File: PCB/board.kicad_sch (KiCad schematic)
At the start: 171 parts, among them J1 Micro_SD_Card, J10 Conn_01x10, J11 Conn_01x02, J12 Conn_02x04_Odd_Even, J13 Conn_01x02, J14 Conn_01x02, J15 Conn_01x03, J16 Conn_01x02, J17 Conn_01x05, J18 Conn_01x04, J19 Conn_01x04, J2 Conn_ARM_JTAG_SWD_10, J20 Conn_01x02, J21 Conn_01x03, J22 Conn_02x04_Odd_Even, J23 Conn_01x04, J24 Conn_01x04, J25 Conn_01x02, J26 Conn_01x03, J27 Conn_02x04_Odd_Even, J28 Conn_01x04, J29 Conn_01x04, J30 Conn_01x02, J31 Conn_01x03, J32 Conn_01x02, J33 Conn_01x02, J34 Conn_01x02, J35 Conn_01x02, J36 Conn_01x02, J37 Conn_01x02, J4 Conn_01x04, J5 Conn_01x04, J6 Conn_01x02, J7 Conn_01x03, J8 Conn_02x04_Odd_Even, J9 Conn_01x10, P1 USB_C_Plug_USB2.0, Q1 IRLML6402, Q2 NMOS, Q3 NMOS, Q4 NMOS, Q5 NMOS, Q6 NMOS, SW1 SW_SPST, SW2 SW_Push, U1 STM32H743VITx, U2 AMS1117-3.3, U3 TPS54331, U4 TMC2209_SILENTSTEPSTICK, U5 TMC2209_SILENTSTEPSTICK, U6 TMC2209_SILENTSTEPSTICK, U7 TMC2209_SILENTSTEPSTICK, Y1 25 MHz

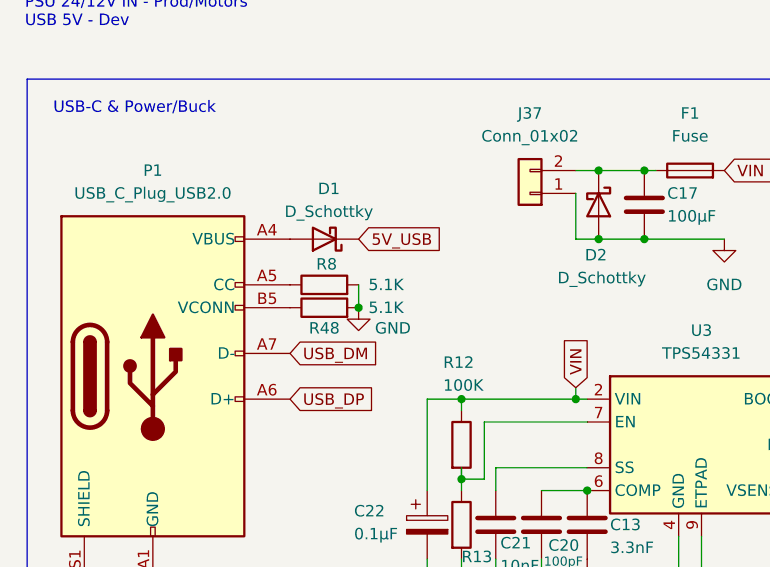
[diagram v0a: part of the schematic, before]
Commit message: A LOT more footprint stuff
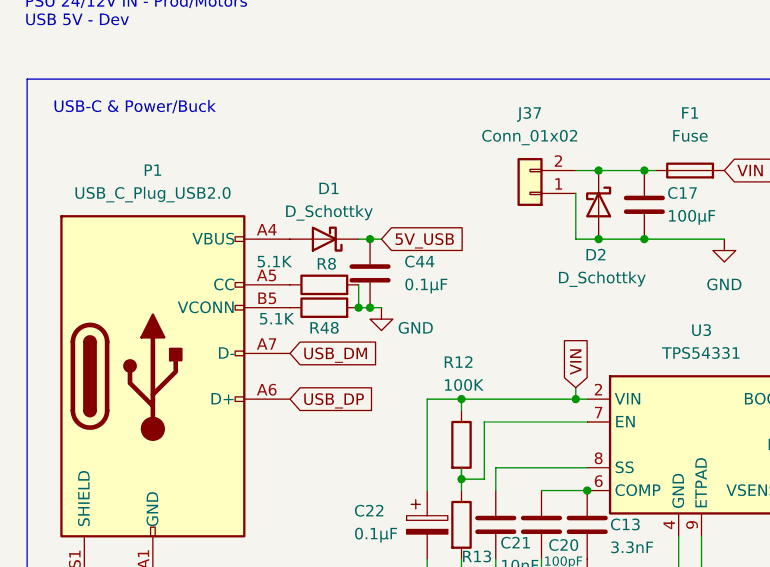
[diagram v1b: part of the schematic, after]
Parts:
- added C44: 0.1µF, Capacitor_SMD:C_0603_1608Metric, symbol Device:C
- D7, R16, R17, R18, R21, R23, R25, R26, R28, R29, R30, R31, R32, R33, R34, R35, R36, R37, R38, R39, R40, R46, R47, R49, R50, R51, R52, R53, R54: footprint (none) -> Resistor_SMD:R_0603_1608Metric
- R14, R15, R9: footprint Resistor_SMD:R_0603_1608Metric -> Resistor_SMD:R_0805_2012Metric
- R20, R22, R24, R27: footprint (none) -> Resistor_SMD:R_0805_2012Metric
- R48, R8: footprint Resistor_SMD:R_0402_1005Metric -> Resistor_SMD:R_0603_1608Metric
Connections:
- net 5V_USB: now also C44.1
- net GND: now also C44.2
